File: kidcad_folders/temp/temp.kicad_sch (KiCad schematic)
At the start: 5 parts, among them SW1 SW_DIP_x01, U1 74LS76

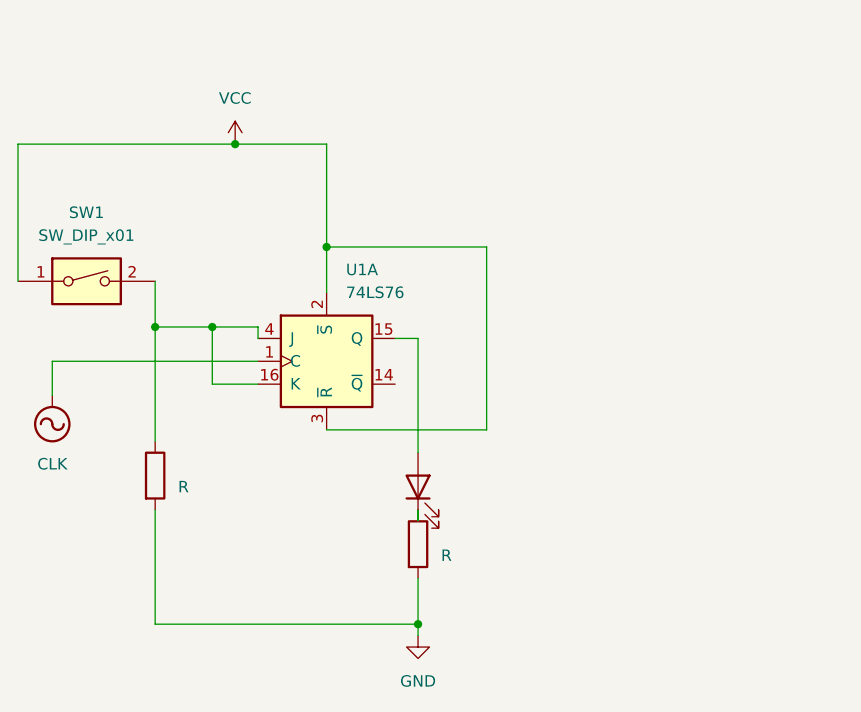
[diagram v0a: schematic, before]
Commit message: push
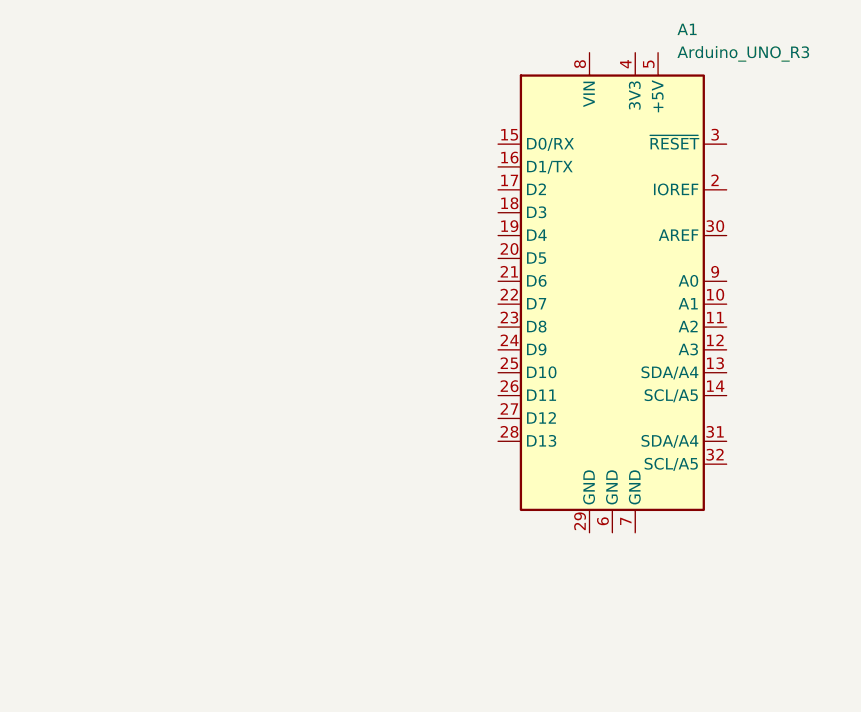
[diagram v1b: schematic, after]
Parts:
- removed D7: LED, symbol Device:LED
- removed R4, R5: R, symbol Device:R
- removed SW1: SW_DIP_x01, symbol Switch:SW_DIP_x01
- removed U1: 74LS76, symbol 74xx:74LS76
- added A1: Arduino_UNO_R3, Module:Arduino_UNO_R3, symbol MCU_Module:Arduino_UNO_R3
